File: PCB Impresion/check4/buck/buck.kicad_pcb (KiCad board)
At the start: 2 copper layers, 45.5 x 36.5 mm, 8 parts, among them J1 OUT, J2 OUT, J3 OUT, Q1 IRF3205, Q2 IRF3205

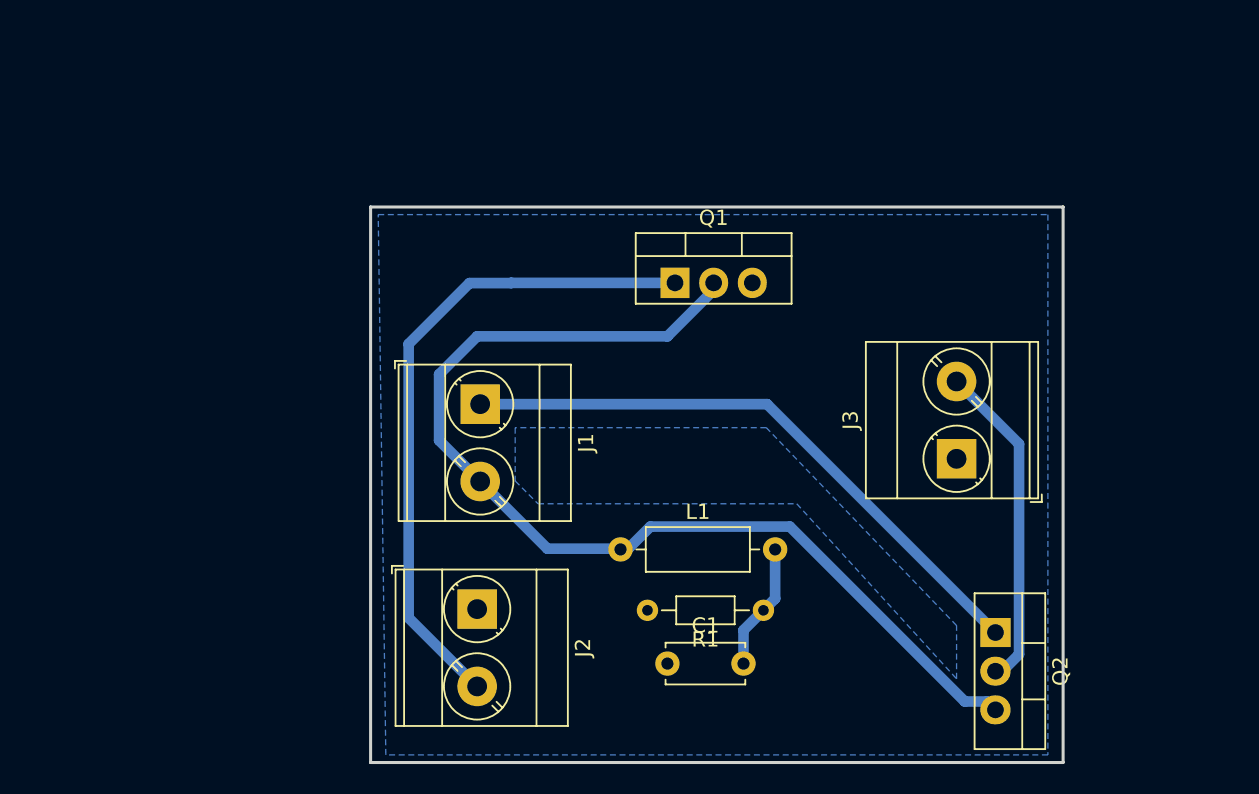
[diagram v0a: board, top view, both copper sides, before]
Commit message: pcb buck
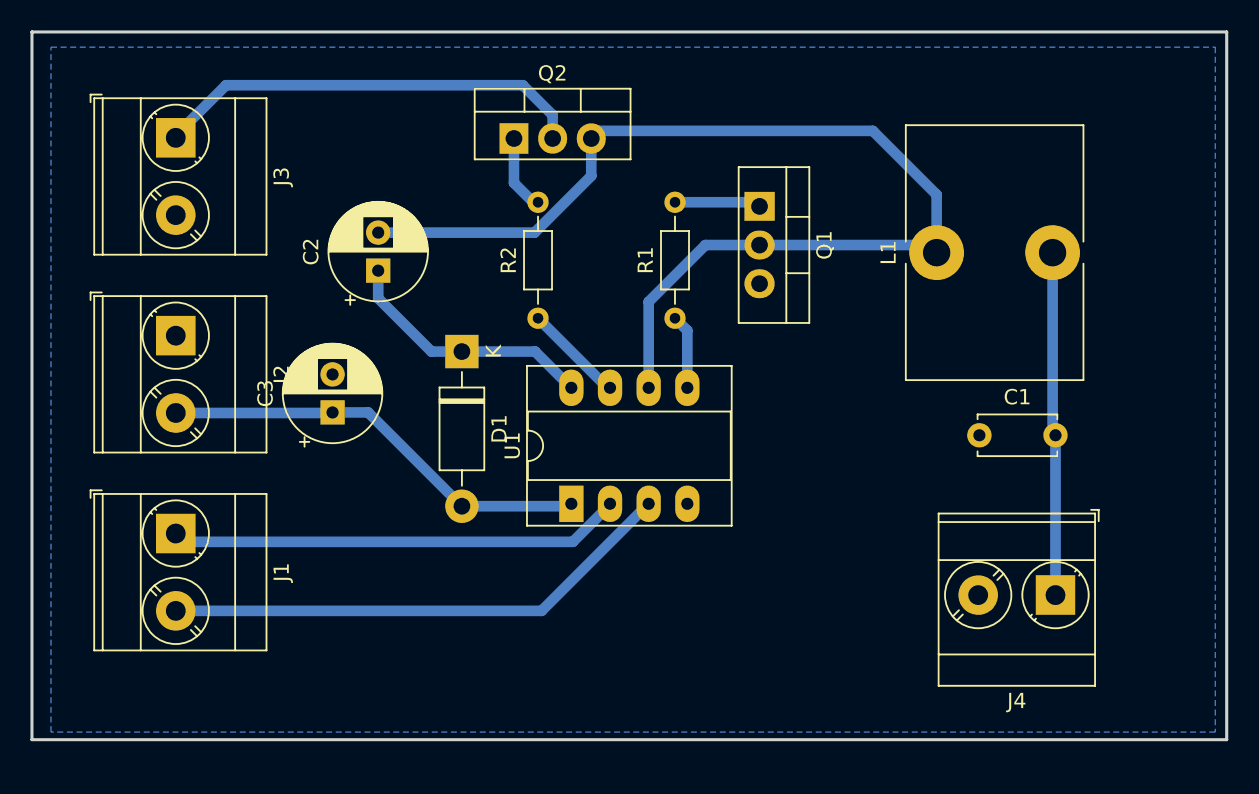
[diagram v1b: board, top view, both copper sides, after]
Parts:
- added C2: 22u, Capacitor_THT:CP_Radial_D6.3mm_P2.50mm, F.Cu at (107.0, 81.2)
- added C3: 10u, Capacitor_THT:CP_Radial_D6.3mm_P2.50mm, F.Cu at (104.0, 90.5)
- added D1: 1N5819, Diode_THT:D_DO-41_SOD81_P10.16mm_Horizontal, F.Cu at (112.5, 86.5)
- added J4: OUT, TerminalBlock_Phoenix:TerminalBlock_Phoenix_MKDS-3-2-5.08_1x02_P5.08mm_Horizontal, F.Cu at (151.5, 102.5)
- added R2: 10, Resistor_THT:R_Axial_DIN0204_L3.6mm_D1.6mm_P7.62mm_Horizontal, F.Cu at (117.5, 84.3)
- added U1: IR2104, Package_DIP:CERDIP-8_W7.62mm_SideBrazed_LongPads_Socket, F.Cu at (119.7, 96.5)
- C1: value 1u -> 2.7u
- J1: value OUT -> V
- J2: value OUT -> VCC
- J3: value OUT -> VIN
- L1: value 1m -> 200u; footprint Inductor_THT:L_Axial_L6.6mm_D2.7mm_P10.16mm_Horizontal_Vishay_IM-2 -> Inductor_THT:L_Toroid_Vertical_L16.5mm_W11.4mm_P7.62mm_Pulse_KM-2
- R1: value 22K -> 10
- moved J3 55.5 mm to (93.7, 72.5), turned to -90 degrees
- moved Q2 45.3 mm to (115.9, 72.5), turned to 0 degrees
- moved L1 28.5 mm to (143.7, 80.0), turned to 90 degrees
- moved J2 26.7 mm to (93.7, 85.5)
- moved C1 25.4 mm to (146.5, 92.0)
- moved J1 21.7 mm to (93.7, 98.5)
- moved R1 20.1 mm to (126.5, 84.3), turned to 90 degrees
- moved Q1 7.49 mm to (132.1, 77.0), turned to -90 degrees
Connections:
- C1 pad 2: Net-(C1-Pad2) -> Net-(J4-Pin_1)
- J1 pad 1: Net-(J1-Pin_1) -> Net-(J1-Pin_2)
- J1 pad 2: Net-(J1-Pin_2) -> Net-(J1-Pin_1)
- J2 pad 2: Net-(J2-Pin_2) -> Vcc
- L1 pad 1: Net-(J1-Pin_2) -> Vs
- L1 pad 2: Net-(C1-Pad2) -> Net-(J4-Pin_1)
- Q1 pad 1: Net-(J2-Pin_2) -> Lo
- Q1 pad 2: Net-(J1-Pin_2) -> Vs
- Q2 pad 1: Net-(J1-Pin_1) -> Ho
- Q2 pad 3: Net-(J1-Pin_2) -> Vs
- R1 pad 1: Net-(C1-Pad2) -> Net-(U1-LO)
- R1 pad 2: GND -> Lo
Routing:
- net Vs: track 0.00 -> 72.8 mm
- net Net-(J2-Pin_2): track 43.5 -> 0.00 mm
- net Net-(J1-Pin_2): track 70.7 -> 29.8 mm
- net Vcc: track 0.00 -> 28.6 mm
- net Net-(J4-Pin_1): track 0.00 -> 22.6 mm
- net Net-(D1-K): track 0.00 -> 16.9 mm
- net Net-(C1-Pad2): track 8.36 -> 0.00 mm
- net Net-(J3-Pin_2): track 21.6 -> 28.6 mm
- net Net-(U1-HO): track 0.00 -> 6.62 mm
- net Net-(J1-Pin_1): track 40.1 -> 34.0 mm
- net Lo: track 0.00 -> 5.67 mm
- net Ho: track 0.00 -> 5.03 mm
- net Net-(U1-LO): track 0.00 -> 4.91 mm
- removed copper zone on B.Cu, net (none)
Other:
- board size 45.5 x 36.5 mm -> 78.5 x 46.5 mm
